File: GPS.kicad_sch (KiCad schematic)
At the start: 15 parts, among them J29 Conn_01x05, U12 AMS1117-3.3, U42 2.54mm 1x6 socket, U43 2.54mm 1x8 socket, U44 2.54mm 1x8 socket, U45 2.54mm 1x10 socket, U46 2.54mm 2x6 socket

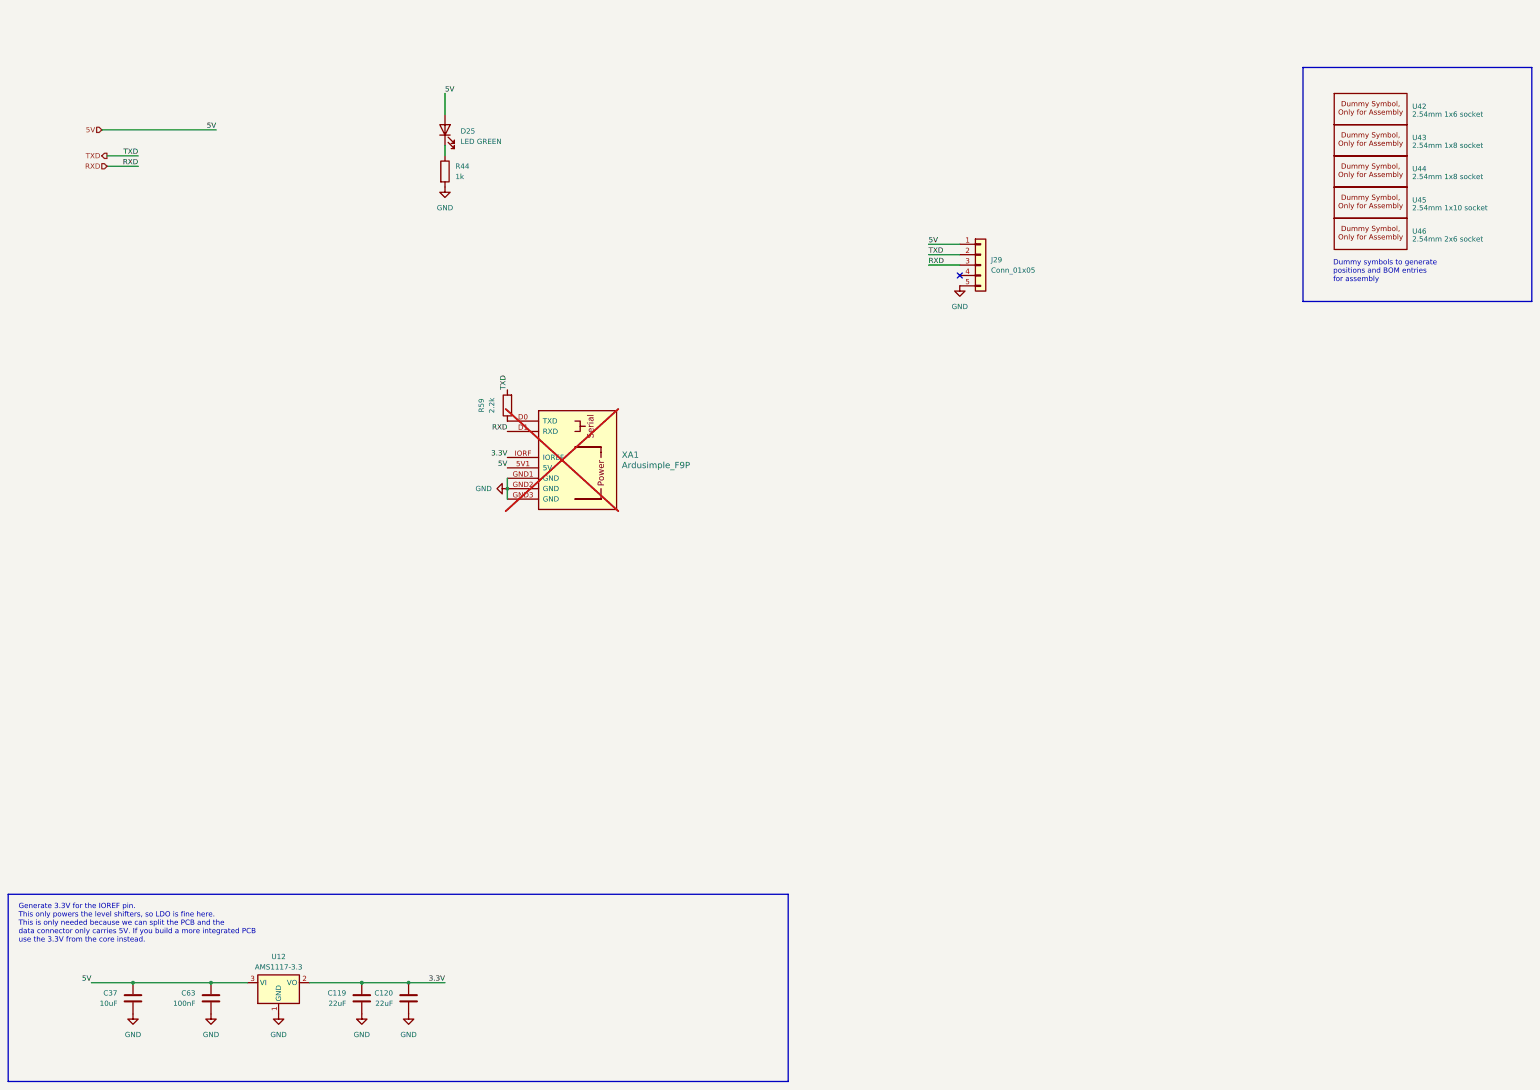
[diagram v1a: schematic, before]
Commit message: Routing progress
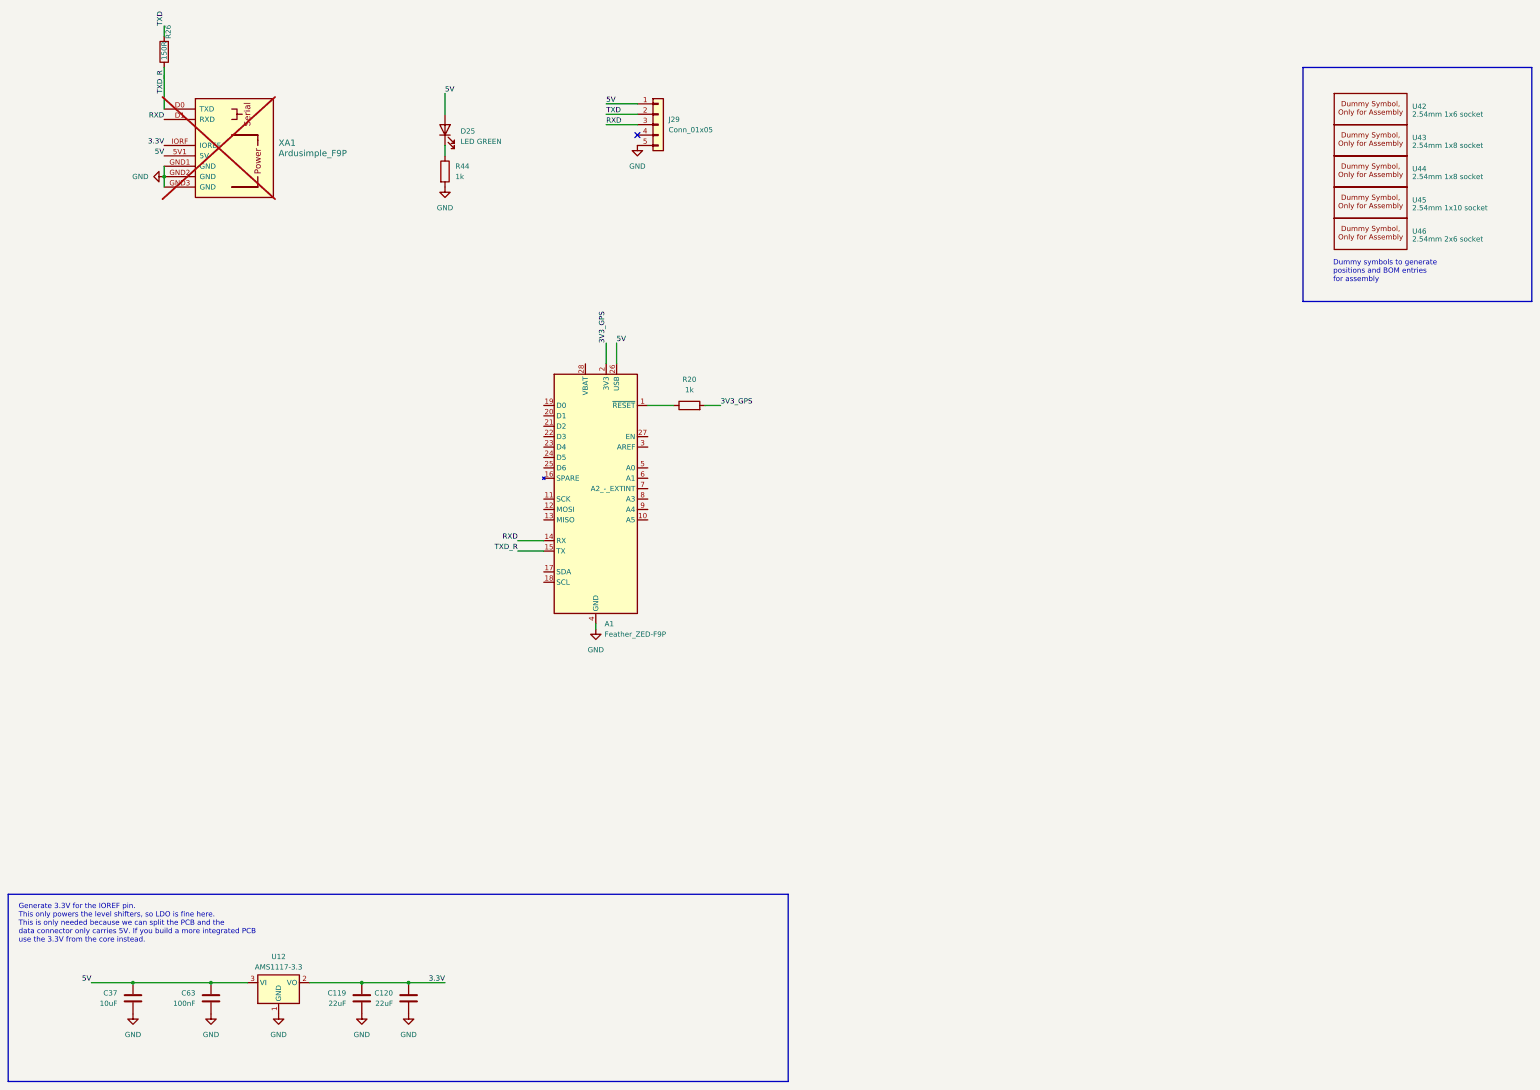
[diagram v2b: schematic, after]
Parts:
- removed R59: 2.2k, Resistor_SMD:R_0805_2012Metric, symbol Device:R
- added A1: Feather_ZED-F9P, Module:Adafruit_Feather_WithMountingHoles, symbol GNSS_layberge:Feather_ZED-F9P
- added R20: 1k, Resistor_SMD:R_0805_2012Metric, symbol Device:R
- added R26: 150R, Resistor_SMD:R_0603_1608Metric, symbol Device:R
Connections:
- net 5V: now also A1.26 (USB)
- net GND: now also A1.4 (GND)
- net RXD: now also A1.14 (RX)
- net TXD: now also R26.2
- net TXD_R: now reaches XA1.D0 (TXD)
- net TXD_R: now also A1.15 (TX), R26.1
- new net: A1.1 (~{RESET}), R20.1
- new net 3V3_GPS: A1.2 (3V3), R20.2
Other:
- moved on the sheet: J29, XA1
